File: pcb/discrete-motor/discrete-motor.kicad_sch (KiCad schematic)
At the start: 28 parts

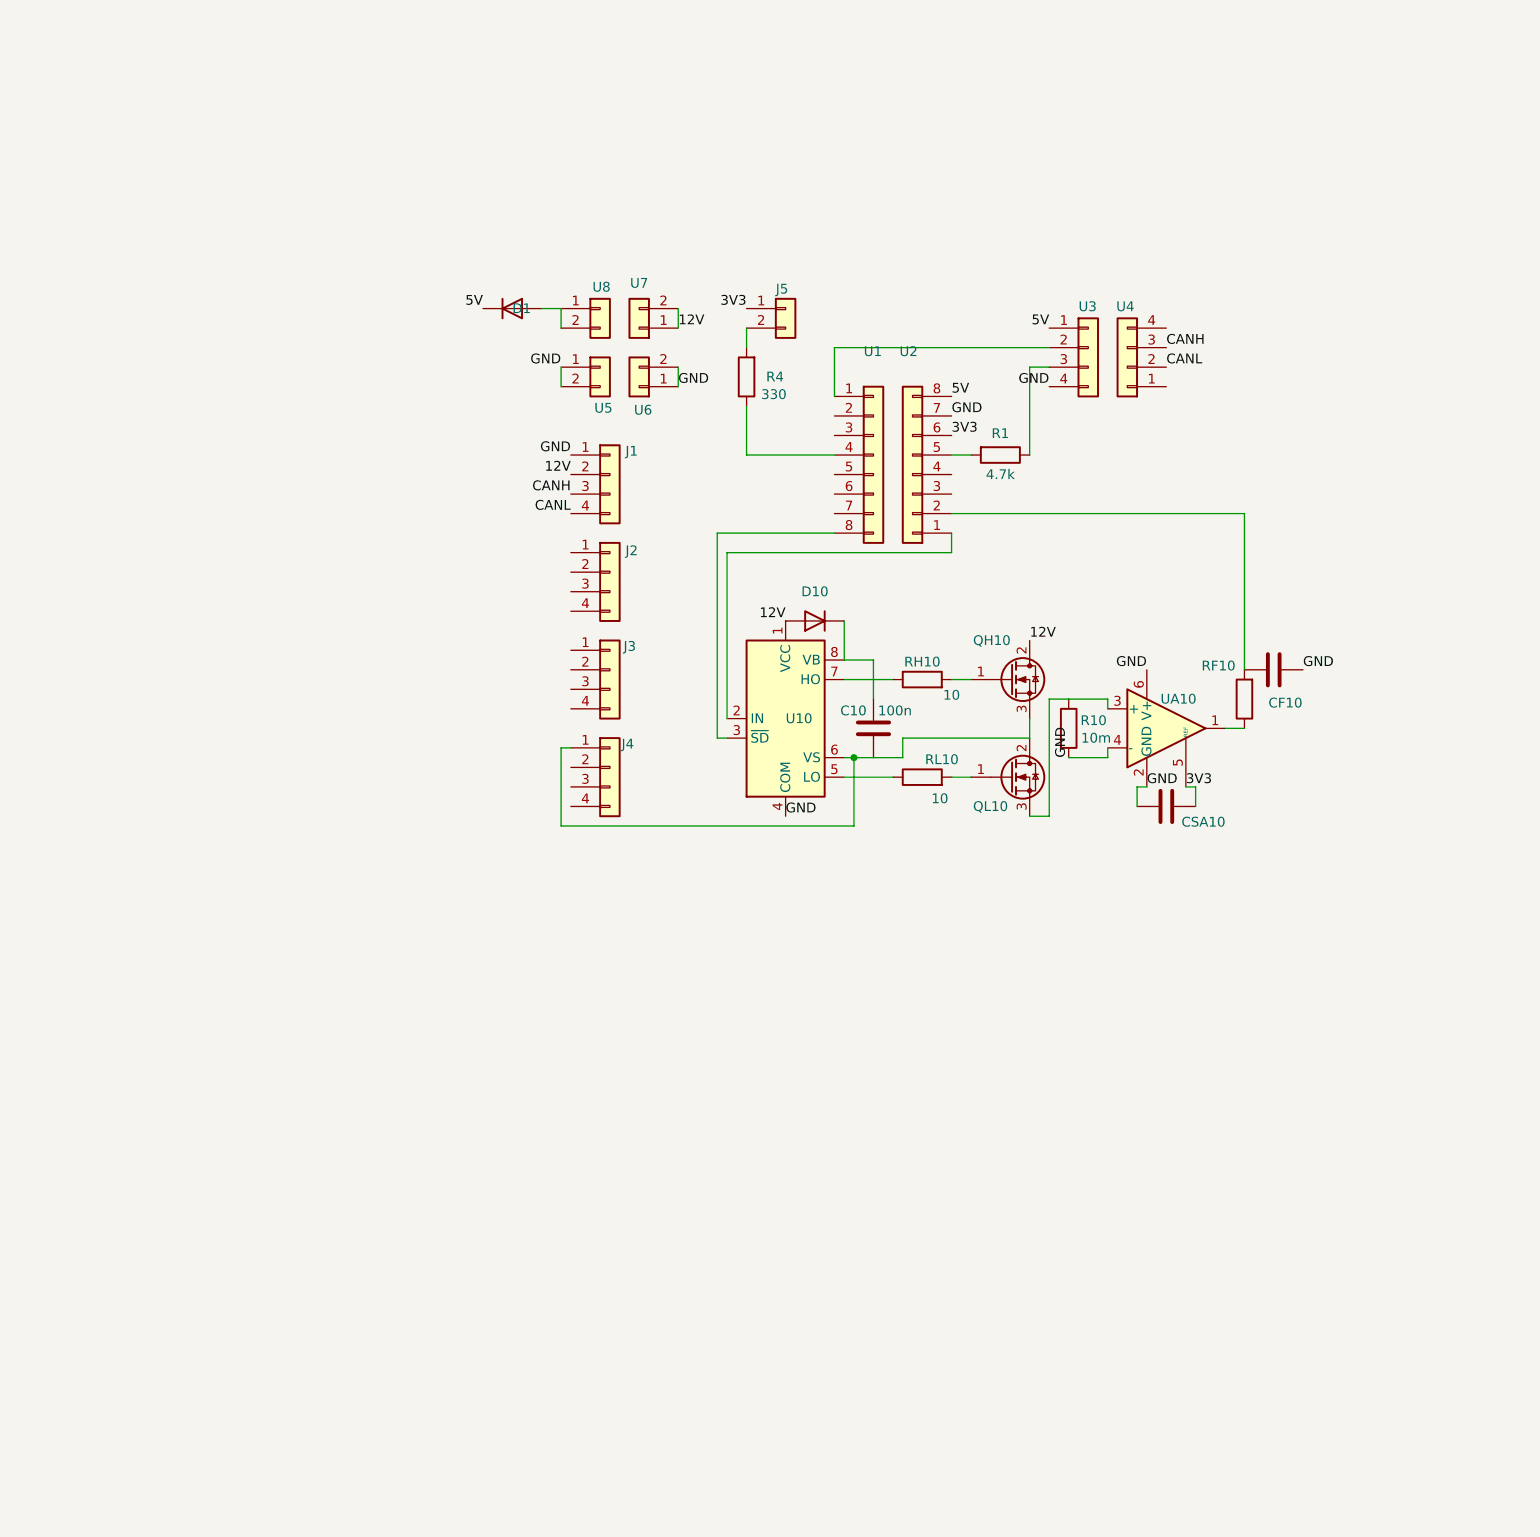
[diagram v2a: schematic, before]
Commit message: discrete motor
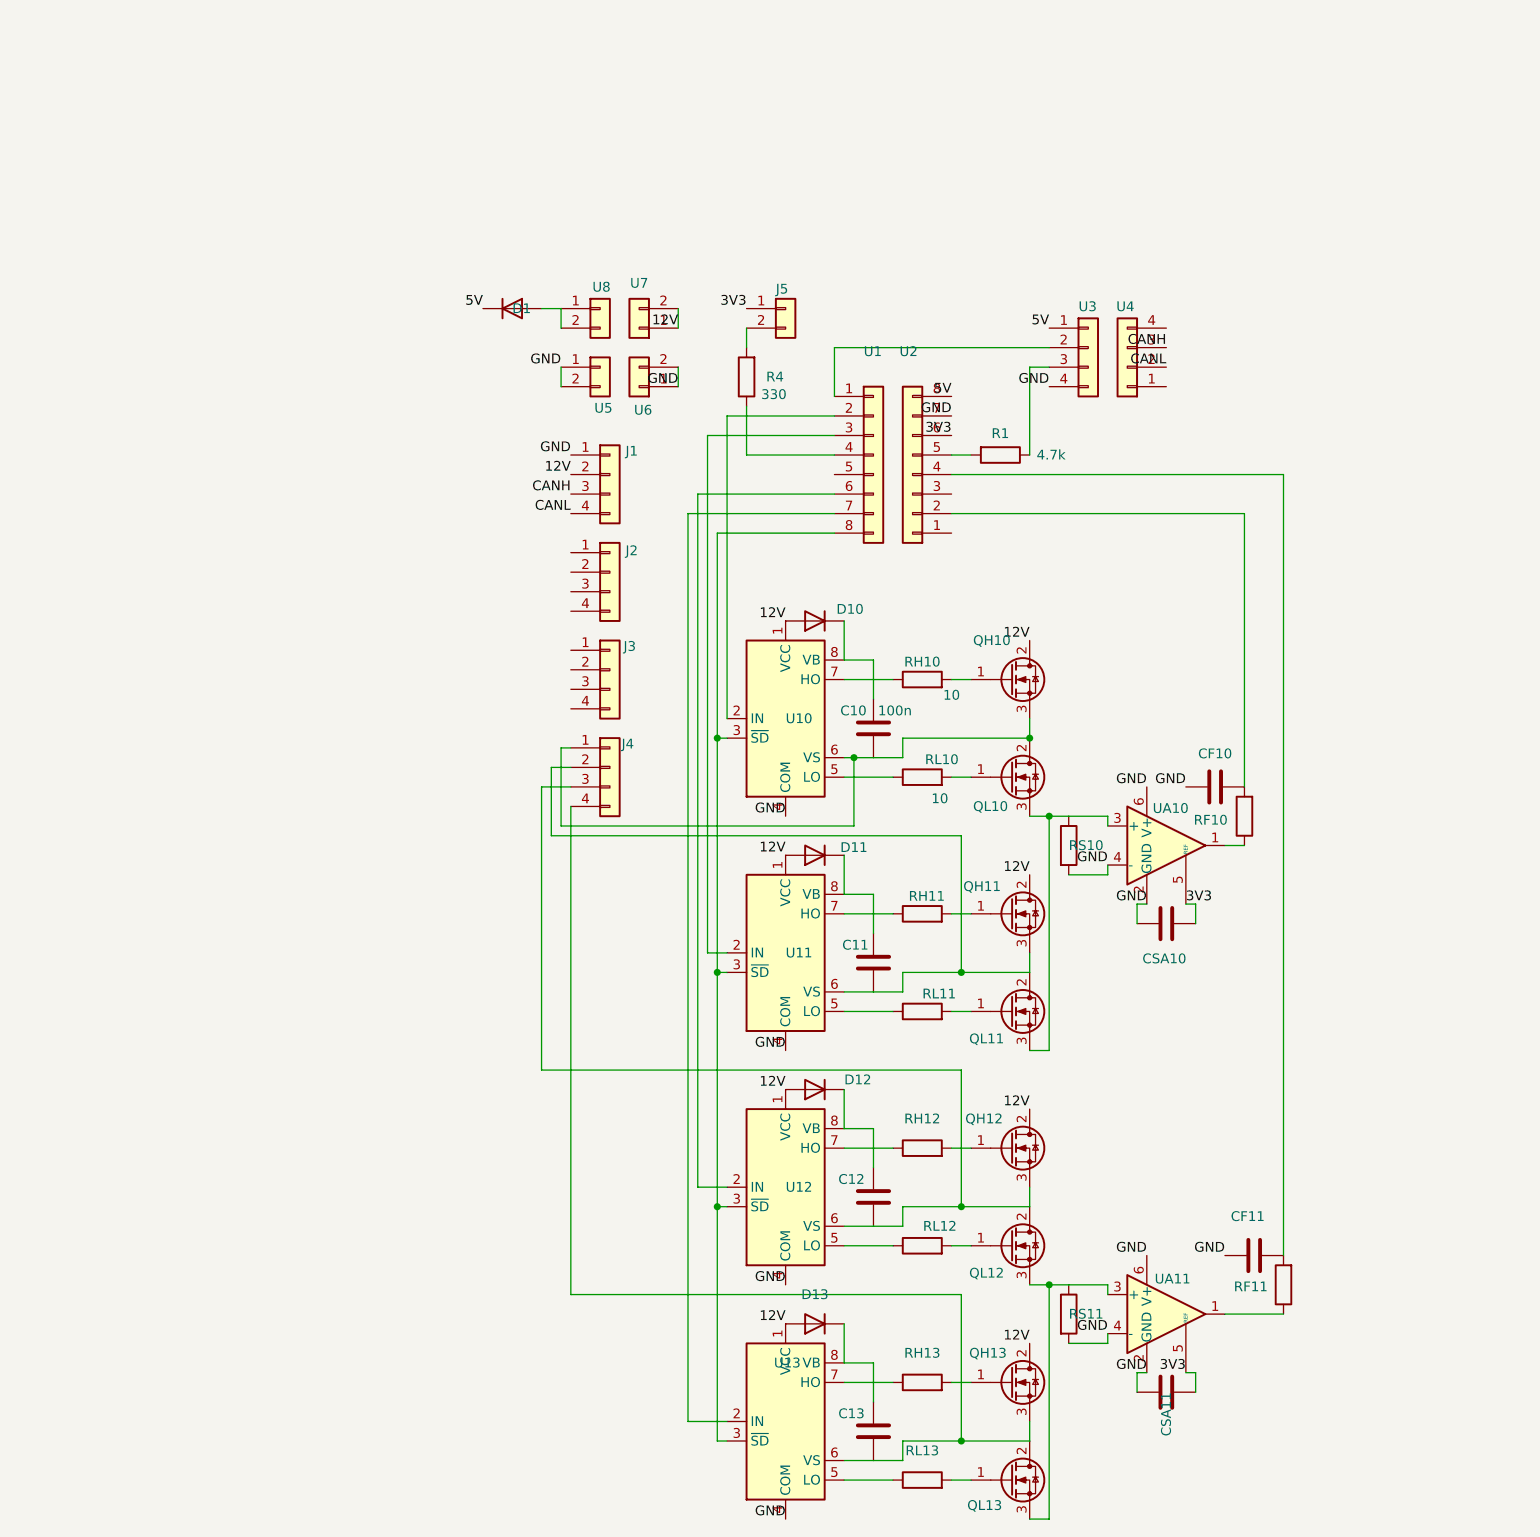
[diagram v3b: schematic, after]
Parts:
- removed R10: 10m, Resistor_SMD:R_1206_3216Metric, symbol Device:R
- added C11, C12, C13, CF11, CSA11: 100n, Capacitor_SMD:C_0603_1608Metric, symbol Device:C
- added D11, D12, D13: ~, Diode_SMD:D_SMA, symbol Device:D
- added QH11, QH12, QH13, QL11, QL12, QL13: ~, Package_TO_SOT_SMD:TO-263-2, symbol Transistor_FET:Q_NMOS_GDS
- added RF11: 1k, Resistor_SMD:R_0603_1608Metric, symbol Device:R
- added RH11, RH12, RH13, RL11, RL12, RL13: 10, Resistor_SMD:R_0603_1608Metric, symbol Device:R
- added RS10, RS11: 10m, Resistor_SMD:R_1206_3216Metric, symbol Device:R
- added U11, U12, U13: ~, Package_SO:SOIC-8_3.9x4.9mm_P1.27mm, symbol Driver_FET:IR2104
- added UA11: ~, Package_TO_SOT_SMD:SOT-23-6, symbol Amplifier_Current:INA181
- D1, D10, J1, J2, J3, J4, J5, U1, U2, U3, U4, U5, U6, U7, U8, UA10: value (none) -> ~
- QH10, QL10: value (none) -> ~; footprint fixme!!! -> Package_TO_SOT_SMD:TO-263-2; lcsc (none) -> C409762
- U10: value (none) -> ~; footprint Package_SO:SOIC-8 -> Package_SO:SOIC-8_3.9x4.9mm_P1.27mm; lcsc (none) -> C5804631
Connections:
- net 12V: now also D11.2 (A), D12.2 (A), D13.2 (A), QH11.2 (D), QH12.2 (D), QH13.2 (D), U11.1 (VCC), U12.1 (VCC), U13.1 (VCC)
- net 3V3: now also CSA11.1, UA11.5 (REF)
- net GND: now also CF11.2, CSA11.2, RS10.2, RS11.2, U11.4 (COM), U12.4 (COM), U13.4 (COM), UA11.2 (GND), UA11.4 (-), UA11.6 (V+)
- net at U2.1 (Pin_1): no longer U10.2 (IN)
- net at U2.4 (Pin_4): now also CF11.1, RF11.2
- net at J4.2 (Pin_2): now also C11.2, QH11.3 (S), QL11.2 (D), U11.6 (VS)
- net at J4.3 (Pin_3): now also C12.2, QH12.3 (S), QL12.2 (D), U12.6 (VS)
- net at J4.4 (Pin_4): now also C13.2, QH13.3 (S), QL13.2 (D), U13.6 (VS)
- net at QL10.3 (S), UA10.3 (+): now also QL11.3 (S), RS10.1
- net at U1.2 (Pin_2): now also U10.2 (IN)
- net at U1.3 (Pin_3): now also U11.2 (IN)
- net at U1.6 (Pin_6): now also U12.2 (IN)
- net at U1.7 (Pin_7): now also U13.2 (IN)
- net at U1.8 (Pin_8), U10.3 (~{SD}): now also U11.3 (~{SD}), U12.3 (~{SD}), U13.3 (~{SD})
- new net: C12.1, D12.1 (K), U12.8 (VB)
- new net: C13.1, D13.1 (K), U13.8 (VB)
- new net: QL11.1 (G), RL11.2
- new net: C11.1, D11.1 (K), U11.8 (VB)
- new net: QL12.1 (G), RL12.2
- new net: QL12.3 (S), QL13.3 (S), RS11.1, UA11.3 (+)
- new net: RL11.1, U11.5 (LO)
- new net: RH11.1, U11.7 (HO)
- new net: RL13.1, U13.5 (LO)
- new net: RH13.1, U13.7 (HO)
- new net: QH13.1 (G), RH13.2
- new net: RF11.1, UA11.1
- new net: QH11.1 (G), RH11.2
- new net: QL13.1 (G), RL13.2
- new net: QH12.1 (G), RH12.2
- new net: RL12.1, U12.5 (LO)
- new net: RH12.1, U12.7 (HO)

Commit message: pcb wip
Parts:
- C10, C11, C12, C13, CF10, CF11, CSA10, CSA11: lcsc C53084461 -> C1590
- D1, D10, D11, D12, D13, J1, J2, J3, J4, J5, U1, U2, U3, U4, U5, U6, U7, U8, UA10, UA11: value ~ -> (none)
- QH10, QH11, QH12, QH13, QL10, QL11, QL12, QL13: value ~ -> (none); lcscRot (none) -> 180
- RH10, RH11, RH12, RH13, RL10, RL11, RL12, RL13: footprint Resistor_SMD:R_0603_1608Metric -> Resistor_SMD:R_0402_1005Metric
- U10, U11, U12, U13: value ~ -> (none); lcscRot (none) -> -90
